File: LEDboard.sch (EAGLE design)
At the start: 307 parts, among them IC1 REG1117, Q1 MMUN2133LT1G, U1 IS31FL3741_QFN60, U2 IS31FL3741_QFN60, U3 ATSAMD21G-A, U4 TPS61090RSAR, U5 MCP73831T-2ACI/OT

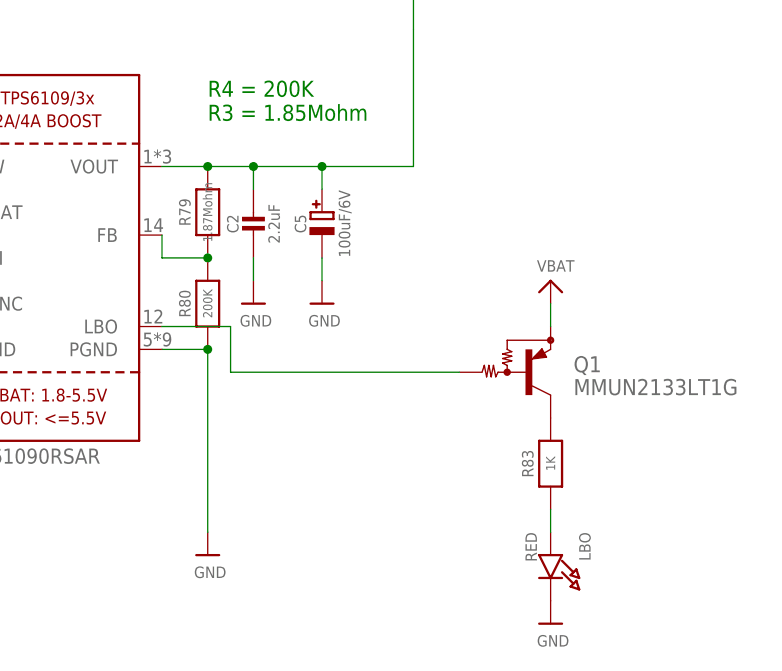
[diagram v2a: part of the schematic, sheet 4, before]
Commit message: Remove LBO, change bypass cap
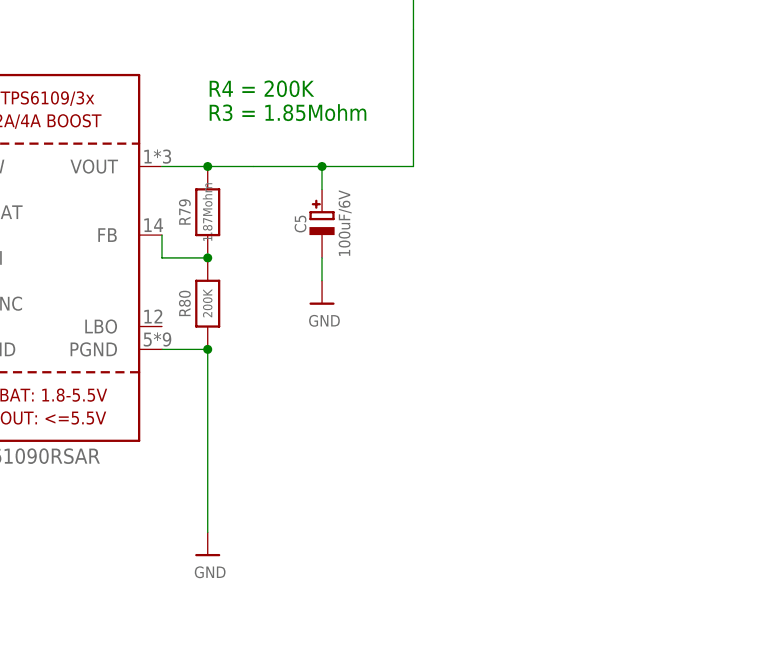
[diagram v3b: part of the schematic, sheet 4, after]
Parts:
- removed C2: 2.2uF, microbuilder:CAP_CERAMIC0805-NOOUTLINE
- removed LBO: RED, microbuilder:LED0805_NOOUTLINE
- removed Q1: MMUN2133LT1G, transistor:MUN2114T1-PNP_DRIVER-SC59-BEC
- removed R83: 1K, microbuilder:RESISTOR0805_NOOUTLINE
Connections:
- removed net LBO: Q1.B, U4.LBO
- removed net N$77: LBO.A, R83.1
- removed net N$78: Q1.C, R83.2
- net 5.0V: no longer C2.1
- net GND: no longer C2.2, LBO.C
- net VBAT: no longer Q1.E
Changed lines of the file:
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@@
 <part name="B1" library="microbuilder" deviceset="BATTERY" device="" value="S2B-PH-SM4-TB(LF)(SN)"/>
 <part name="U$5" library="microbuilder" deviceset="GND" device=""/>
-<part name="C2" library="microbuilder" deviceset="CAP_CERAMIC" device="0805-NOOUTLINE" value="2.2uF"/>
 <part name="U$7" library="microbuilder" deviceset="5.0V" device=""/>
 <part name="U$19" library="microbuilder" deviceset="VBAT" device=""/>
@@
 <part name="R80" library="microbuilder" deviceset="RESISTOR" device="0805_NOOUTLINE" value="200K"/>
 <part name="U$3" library="microbuilder" deviceset="GND" device=""/>
-<part name="U$6" library="microbuilder" deviceset="GND" device=""/>
 <part name="U$8" library="microbuilder" deviceset="GND" device=""/>
 <part name="R81" library="microbuilder" deviceset="RESISTOR" device="0805_NOOUTLINE" value="340K"/>
 <part name="R82" library="microbuilder" deviceset="RESISTOR" device="0805_NOOUTLINE" value="1.87Mohm"/>
 <part name="C5" library="microbuilder" deviceset="CAP_TANTALUM" device="B/3528_REFLOW" value="100uF/6V"/>
-<part name="LBO" library="microbuilder" deviceset="LED" device="0805_NOOUTLINE" value="RED"/>
-<part name="R83" library="microbuilder" deviceset="RESISTOR" device="0805_NOOUTLINE" value="1K"/>
-<part name="U$20" library="microbuilder" deviceset="GND" device=""/>
-<part name="U$11" library="microbuilder" deviceset="VBAT" device=""/>
-<part name="Q1" library="transistor" deviceset="*-PNP_DRIVER-" device="SC59-BEC" technology="MUN2114T1" value="MMUN2133LT1G"/>
 <part name="U5" library="microbuilder" deviceset="MCP73831/2" device="" value="MCP73831T-2ACI/OT"/>
 <part name="LED3" library="microbuilder" deviceset="LED" device="0805_NOOUTLINE" value="ORANGE"/>
@@
 <instance part="B1" gate="G$1" x="22.86" y="55.88" rot="R90"/>
 <instance part="U$5" gate="G$1" x="22.86" y="48.26"/>
-<instance part="C2" gate="G$1" x="106.68" y="60.96"/>
 <instance part="U$7" gate="G$1" x="124.46" y="91.44"/>
 <instance part="U$19" gate="G$1" x="38.1" y="73.66"/>
@@
 <instance part="R80" gate="G$1" x="101.6" y="53.34" rot="R90"/>
 <instance part="U$3" gate="G$1" x="101.6" y="25.4"/>
-<instance part="U$6" gate="G$1" x="106.68" y="53.34"/>
 <instance part="U$8" gate="G$1" x="114.3" y="53.34"/>
 <instance part="R81" gate="G$1" x="53.34" y="35.56" rot="R90"/>
 <instance part="R82" gate="G$1" x="53.34" y="58.42" rot="R90"/>
 <instance part="C5" gate="G$1" x="114.3" y="60.96"/>
-<instance part="LBO" gate="G$1" x="139.7" y="22.86" rot="R270"/>
-<instance part="R83" gate="G$1" x="139.7" y="35.56" rot="R90"/>
-<instance part="U$20" gate="G$1" x="139.7" y="17.78"/>
-<instance part="U$11" gate="G$1" x="139.7" y="55.88"/>
-<instance part="Q1" gate="G$1" x="137.16" y="45.72" smashed="yes">
-<attribute name="NAME" x="142.24" y="45.72" size="1.778" layer="95"/>
-<attribute name="VALUE" x="142.24" y="43.18" size="1.778" layer="96"/>
-</instance>
 <instance part="U5" gate="G$1" x="114.3" y="127"/>
 <instance part="LED3" gate="G$1" x="81.28" y="124.46"/>
@@
 </segment>
 <segment>
-<pinref part="C2" gate="G$1" pin="2"/>
-<wire x1="106.68" y1="58.42" x2="106.68" y2="55.88" width="0.1524" layer="91"/>
-<pinref part="U$6" gate="G$1" pin="GND"/>
-</segment>
-<segment>
 <wire x1="114.3" y1="58.42" x2="114.3" y2="55.88" width="0.1524" layer="91"/>
 <pinref part="U$8" gate="G$1" pin="GND"/>
@@
 </segment>
 <segment>
-<pinref part="LBO" gate="G$1" pin="C"/>
-<pinref part="U$20" gate="G$1" pin="GND"/>
-</segment>
-<segment>
 <pinref part="U$30" gate="G$1" pin="GND"/>
 <wire x1="50.8" y1="119.38" x2="55.88" y2="119.38" width="0.1524" layer="91"/>
@@
 <wire x1="114.3" y1="68.58" x2="124.46" y2="68.58" width="0.1524" layer="91"/>
 <wire x1="124.46" y1="68.58" x2="124.46" y2="83.82" width="0.1524" layer="91"/>
-<pinref part="C2" gate="G$1" pin="1"/>
 <wire x1="124.46" y1="83.82" x2="124.46" y2="88.9" width="0.1524" layer="91"/>
-<wire x1="106.68" y1="66.04" x2="106.68" y2="68.58" width="0.1524" layer="91"/>
-<junction x="106.68" y="68.58"/>
 <wire x1="114.3" y1="68.58" x2="114.3" y2="66.04" width="0.1524" layer="91"/>
 <junction x="114.3" y="68.58"/>
@@
 </segment>
 <segment>
-<wire x1="139.7" y1="50.8" x2="139.7" y2="53.34" width="0.1524" layer="91"/>
-<pinref part="U$11" gate="G$1" pin="VBAT"/>
-<pinref part="Q1" gate="G$1" pin="E"/>
-</segment>
-<segment>
 <pinref part="U5" gate="G$1" pin="VBAT"/>
 <wire x1="142.24" y1="129.54" x2="127" y2="129.54" width="0.1524" layer="91"/>
@@
 </segment>
 </net>
-<net name="LBO" class="0">
-<segment>
-<pinref part="U4" gate="G$1" pin="LBO"/>
-<wire x1="96.52" y1="50.8" x2="104.14" y2="50.8" width="0.1524" layer="91"/>
-<wire x1="104.14" y1="50.8" x2="104.14" y2="45.72" width="0.1524" layer="91"/>
-<wire x1="104.14" y1="45.72" x2="129.54" y2="45.72" width="0.1524" layer="91"/>
-<pinref part="Q1" gate="G$1" pin="B"/>
-</segment>
-</net>
-<net name="N$77" class="0">
-<segment>
-<pinref part="LBO" gate="G$1" pin="A"/>
-<pinref part="R83" gate="G$1" pin="1"/>
-<wire x1="139.7" y1="27.94" x2="139.7" y2="30.48" width="0.1524" layer="91"/>
-</segment>
-</net>
-<net name="N$78" class="0">
-<segment>
-<pinref part="R83" gate="G$1" pin="2"/>
-<pinref part="Q1" gate="G$1" pin="C"/>
-</segment>
-</net>

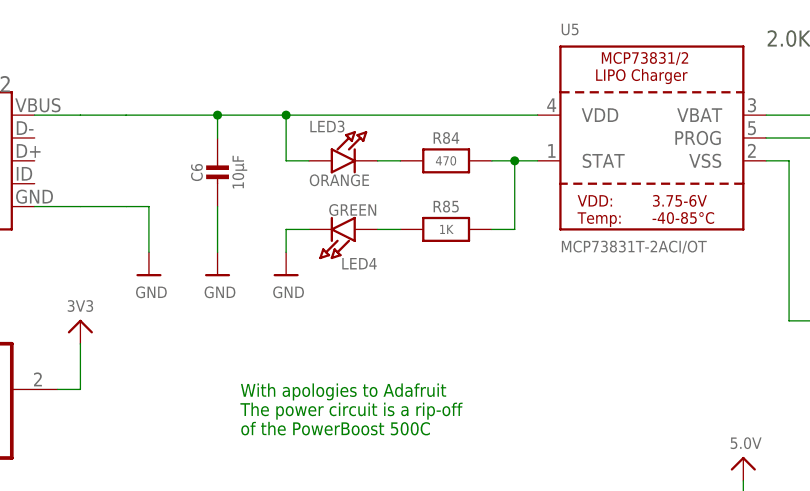
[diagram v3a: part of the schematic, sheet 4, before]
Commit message: holy shit one layer
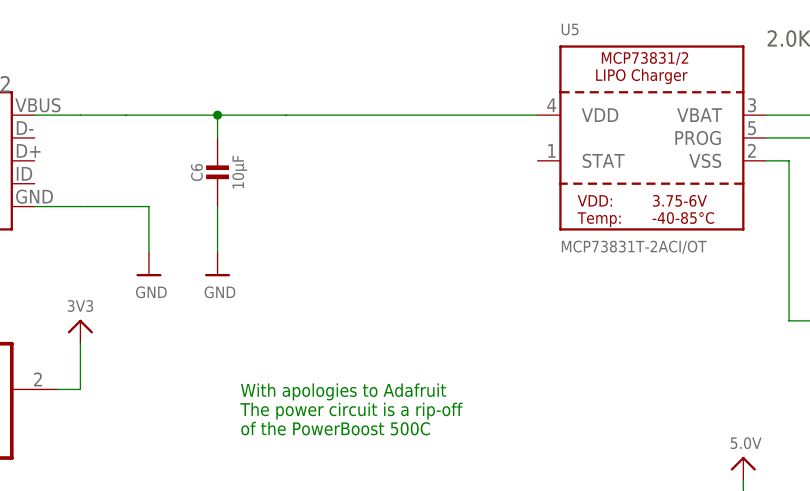
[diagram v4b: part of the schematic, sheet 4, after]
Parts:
- removed LED3: ORANGE, microbuilder:LED0805_NOOUTLINE
- removed LED4: GREEN, microbuilder:LED0805_NOOUTLINE
- removed R84: 470, microbuilder:RESISTOR0805_NOOUTLINE
- removed R85: 1K, microbuilder:RESISTOR0805_NOOUTLINE
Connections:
- removed net N$79: LED3.C, R84.1
- removed net N$80: R84.2, R85.2, U5.STAT
- removed net N$82: LED4.A, R85.1
- net GND: no longer LED4.C
- net VDD1: no longer LED3.A
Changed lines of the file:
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@@
 <part name="C5" library="microbuilder" deviceset="CAP_TANTALUM" device="B/3528_REFLOW" value="100uF/6V"/>
 <part name="U5" library="microbuilder" deviceset="MCP73831/2" device="" value="MCP73831T-2ACI/OT"/>
-<part name="LED3" library="microbuilder" deviceset="LED" device="0805_NOOUTLINE" value="ORANGE"/>
-<part name="LED4" library="microbuilder" deviceset="LED" device="0805_NOOUTLINE" value="GREEN"/>
-<part name="R84" library="microbuilder" deviceset="RESISTOR" device="0805_NOOUTLINE" value="470"/>
-<part name="R85" library="microbuilder" deviceset="RESISTOR" device="0805_NOOUTLINE" value="1K"/>
 <part name="U$30" library="microbuilder" deviceset="GND" device=""/>
 <part name="C6" library="microbuilder" deviceset="CAP_CERAMIC" device="0805-NOOUTLINE" value="10µF"/>
@@
 <part name="R86" library="microbuilder" deviceset="RESISTOR" device="0805_NOOUTLINE" value="2k"/>
 <part name="U$32" library="microbuilder" deviceset="GND" device=""/>
-<part name="U$33" library="microbuilder" deviceset="GND" device=""/>
 <part name="U$34" library="microbuilder" deviceset="VBAT" device=""/>
 <part name="J2" library="SparkFun-Connectors" library_urn="urn:adsk.eagle:library:513" deviceset="USB_MICRO-B" device="_FEMALE-SMT" package3d_urn="urn:adsk.eagle:package:38238/1"/>
@@
 <instance part="C5" gate="G$1" x="114.3" y="60.96"/>
 <instance part="U5" gate="G$1" x="114.3" y="127"/>
-<instance part="LED3" gate="G$1" x="81.28" y="124.46"/>
-<instance part="LED4" gate="G$1" x="78.74" y="116.84" rot="R180"/>
-<instance part="R84" gate="G$1" x="91.44" y="124.46"/>
-<instance part="R85" gate="G$1" x="91.44" y="116.84"/>
 <instance part="U$30" gate="G$1" x="58.42" y="111.76"/>
 <instance part="C6" gate="G$1" x="66.04" y="121.92"/>
@@
 <instance part="R86" gate="G$1" x="137.16" y="127"/>
 <instance part="U$32" gate="G$1" x="142.24" y="101.6"/>
-<instance part="U$33" gate="G$1" x="73.66" y="111.76"/>
 <instance part="U$34" gate="G$1" x="142.24" y="132.08"/>
 <instance part="J2" gate="G$1" x="40.64" y="124.46" rot="MR0"/>
@@
 </segment>
 <segment>
-<pinref part="U$33" gate="G$1" pin="GND"/>
-<wire x1="73.66" y1="116.84" x2="73.66" y2="114.3" width="0.1524" layer="91"/>
-<pinref part="LED4" gate="G$1" pin="C"/>
-<wire x1="76.2" y1="116.84" x2="73.66" y2="116.84" width="0.1524" layer="91"/>
-</segment>
-<segment>
 <wire x1="35.56" y1="86.36" x2="35.56" y2="83.82" width="0.1524" layer="91"/>
 <pinref part="U$10" gate="G$1" pin="GND"/>
@@
 </segment>
 </net>
-<net name="N$79" class="0">
-<segment>
-<pinref part="LED3" gate="G$1" pin="C"/>
-<pinref part="R84" gate="G$1" pin="1"/>
-<wire x1="83.82" y1="124.46" x2="86.36" y2="124.46" width="0.1524" layer="91"/>
-</segment>
-</net>
-<net name="N$80" class="0">
-<segment>
-<pinref part="R84" gate="G$1" pin="2"/>
-<pinref part="U5" gate="G$1" pin="STAT"/>
-<wire x1="96.52" y1="124.46" x2="99.06" y2="124.46" width="0.1524" layer="91"/>
-<pinref part="R85" gate="G$1" pin="2"/>
-<wire x1="99.06" y1="124.46" x2="101.6" y2="124.46" width="0.1524" layer="91"/>
-<wire x1="96.52" y1="116.84" x2="99.06" y2="116.84" width="0.1524" layer="91"/>
-<wire x1="99.06" y1="116.84" x2="99.06" y2="124.46" width="0.1524" layer="91"/>
-<junction x="99.06" y="124.46"/>
-</segment>
-</net>
 <net name="VDD1" class="0">
 <segment>
@@
 <wire x1="66.04" y1="127" x2="66.04" y2="129.54" width="0.1524" layer="91"/>
 <junction x="66.04" y="129.54"/>
-<pinref part="LED3" gate="G$1" pin="A"/>
-<wire x1="76.2" y1="124.46" x2="73.66" y2="124.46" width="0.1524" layer="91"/>
-<wire x1="73.66" y1="124.46" x2="73.66" y2="129.54" width="0.1524" layer="91"/>
-<junction x="73.66" y="129.54"/>
 <pinref part="J2" gate="G$1" pin="VBUS"/>
 <wire x1="45.72" y1="129.54" x2="50.8" y2="129.54" width="0.1524" layer="91"/>
@@
 </segment>
 </net>
-<net name="N$82" class="0">
-<segment>
-<pinref part="R85" gate="G$1" pin="1"/>
-<pinref part="LED4" gate="G$1" pin="A"/>
-<wire x1="86.36" y1="116.84" x2="83.82" y2="116.84" width="0.1524" layer="91"/>
-</segment>
-</net>

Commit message: micro
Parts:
- removed U3: ATSAMD21G-A, SparkFun-IC-Microcontroller:ATSAMD21G-A
- added C1: 1uF, microbuilder:CAP_CERAMIC0805-NOOUTLINE
- added C2: 0.1uF, microbuilder:CAP_CERAMIC0805-NOOUTLINE
- added C3, C4: 10pF, rcl:C-USC0805
- added MCU: ATSAMD21E, adafruit:ATSAMD21E
- added Y1: 32.768kHz, SparkFun-Clocks:CRYSTAL-32.768KHZSMD-3.2X1.5
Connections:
- new net D+: J2.D+, MCU.D+
- new net D-: J2.D-, MCU.D-
- new net N$75: C1.2, MCU.VCORE
- new net N$77: C2.2, MCU.VDD
- new net N$78: C4.1, MCU.PA1, Y1.1
- new net N$79: C3.1, MCU.PA0, Y1.2
- new net RESET: MCU.RESET
- new net SWCLK: MCU.SWCLK
- new net SWDIO: MCU.SWDIO
- net 3V3: now also C1.1, C2.1
- net GND: now also C3.2, C4.2, MCU.GND
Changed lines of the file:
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@@
 <part name="R71" library="SparkFun-Resistors" library_urn="urn:adsk.eagle:library:532" deviceset="14KOHM" device="-0603-1/10W-1%" package3d_urn="urn:adsk.eagle:package:39650/1" value="20Ω"/>
 <part name="R72" library="SparkFun-Resistors" library_urn="urn:adsk.eagle:library:532" deviceset="14KOHM" device="-0603-1/10W-1%" package3d_urn="urn:adsk.eagle:package:39650/1" value="20Ω"/>
-<part name="U3" library="SparkFun-IC-Microcontroller" library_urn="urn:adsk.eagle:library:525" deviceset="ATSAMD21G" device="-A" package3d_urn="urn:adsk.eagle:package:38963/1"/>
 <part name="U4" library="microbuilder" deviceset="VREG_TPS6103X" device="" value="TPS61090RSAR"/>
 <part name="L1" library="microbuilder" deviceset="INDUCTOR" device="TDK_VLC5045" value="VLC5045-6.8uH"/>
@@
 <part name="U$12" library="microbuilder" deviceset="5.0V" device=""/>
 <part name="U$13" library="microbuilder" deviceset="5.0V" device="" value="3V3"/>
+<part name="MCU" library="adafruit" deviceset="ATSAMD21E" device=""/>
+<part name="U$6" library="microbuilder" deviceset="5.0V" device="" value="3V3"/>
+<part name="C1" library="microbuilder" deviceset="CAP_CERAMIC" device="0805-NOOUTLINE" value="1uF"/>
+<part name="U$9" library="microbuilder" deviceset="GND" device=""/>
+<part name="C2" library="microbuilder" deviceset="CAP_CERAMIC" device="0805-NOOUTLINE" value="0.1uF"/>
+<part name="Y1" library="SparkFun-Clocks" library_urn="urn:adsk.eagle:library:511" deviceset="CRYSTAL-32.768KHZ" device="SMD-3.2X1.5" package3d_urn="urn:adsk.eagle:package:37548/1" value="32.768kHz"/>
+<part name="U$11" library="microbuilder" deviceset="GND" device=""/>
+<part name="C3" library="rcl" library_urn="urn:adsk.eagle:library:334" deviceset="C-US" device="C0805" package3d_urn="urn:adsk.eagle:package:23617/2" value="10pF"/>
+<part name="C4" library="rcl" library_urn="urn:adsk.eagle:library:334" deviceset="C-US" device="C0805" package3d_urn="urn:adsk.eagle:package:23617/2" value="10pF"/>
 </parts>
 <sheets>
@@
 </plain>
 <instances>
-<instance part="U3" gate="G$1" x="40.64" y="38.1"/>
+<instance part="MCU" gate="G$1" x="50.8" y="48.26"/>
+<instance part="U$6" gate="G$1" x="22.86" y="81.28"/>
+<instance part="C1" gate="G$1" x="27.94" y="66.04" rot="R90"/>
+<instance part="U$9" gate="G$1" x="22.86" y="10.16"/>
+<instance part="C2" gate="G$1" x="30.48" y="71.12" rot="R90"/>
+<instance part="Y1" gate="G$1" x="78.74" y="50.8" rot="R180"/>
+<instance part="U$11" gate="G$1" x="78.74" y="35.56"/>
+<instance part="C3" gate="G$1" x="73.66" y="45.72"/>
+<instance part="C4" gate="G$1" x="83.82" y="45.72"/>
 </instances>
 <busses>
 </busses>
 <nets>
+<net name="D-" class="0">
+<segment>
+<pinref part="MCU" gate="G$1" pin="D-"/>
+<wire x1="33.02" y1="35.56" x2="22.86" y2="35.56" width="0.1524" layer="91"/>
+<label x="22.86" y="35.56" size="1.778" layer="95"/>
+</segment>
+</net>
+<net name="D+" class="0">
+<segment>
+<pinref part="MCU" gate="G$1" pin="D+"/>
+<wire x1="33.02" y1="38.1" x2="22.86" y2="38.1" width="0.1524" layer="91"/>
+<label x="22.86" y="38.1" size="1.778" layer="95"/>
+</segment>
+</net>
+<net name="3V3" class="0">
+<segment>
+<pinref part="U$6" gate="G$1" pin="5.0V"/>
+<wire x1="22.86" y1="73.66" x2="22.86" y2="78.74" width="0.1524" layer="91"/>
+<wire x1="22.86" y1="71.12" x2="22.86" y2="73.66" width="0.1524" layer="91"/>
+<pinref part="C1" gate="G$1" pin="1"/>
+<wire x1="22.86" y1="66.04" x2="22.86" y2="71.12" width="0.1524" layer="91"/>
+<pinref part="C2" gate="G$1" pin="1"/>
+<wire x1="25.4" y1="71.12" x2="22.86" y2="71.12" width="0.1524" layer="91"/>
+<junction x="22.86" y="71.12"/>
+</segment>
+</net>
+<net name="N$75" class="0">
+<segment>
+<pinref part="MCU" gate="G$1" pin="VCORE"/>
+<pinref part="C1" gate="G$1" pin="2"/>
+<wire x1="33.02" y1="66.04" x2="30.48" y2="66.04" width="0.1524" layer="91"/>
+</segment>
+</net>
+<net name="GND" class="0">
+<segment>
+<wire x1="22.86" y1="15.24" x2="22.86" y2="12.7" width="0.1524" layer="91"/>
+<pinref part="U$9" gate="G$1" pin="GND"/>
+<pinref part="MCU" gate="G$1" pin="GND"/>
+<wire x1="33.02" y1="15.24" x2="22.86" y2="15.24" width="0.1524" layer="91"/>
+</segment>
+<segment>
+<wire x1="78.74" y1="40.64" x2="78.74" y2="38.1" width="0.1524" layer="91"/>
+<pinref part="U$11" gate="G$1" pin="GND"/>
+<pinref part="C3" gate="G$1" pin="2"/>
+<wire x1="73.66" y1="40.64" x2="78.74" y2="40.64" width="0.1524" layer="91"/>
+<pinref part="C4" gate="G$1" pin="2"/>
+<wire x1="83.82" y1="40.64" x2="78.74" y2="40.64" width="0.1524" layer="91"/>
+<junction x="78.74" y="40.64"/>
+</segment>
+</net>
+<net name="N$77" class="0">
+<segment>
+<pinref part="C2" gate="G$1" pin="2"/>
+<pinref part="MCU" gate="G$1" pin="VDD"/>
+</segment>
+</net>
+<net name="N$78" class="0">
+<segment>
+<pinref part="MCU" gate="G$1" pin="PA1"/>
+<wire x1="63.5" y1="53.34" x2="81.28" y2="53.34" width="0.1524" layer="91"/>
+<pinref part="Y1" gate="G$1" pin="1"/>
+<wire x1="81.28" y1="53.34" x2="81.28" y2="50.8" width="0.1524" layer="91"/>
+<pinref part="C4" gate="G$1" pin="1"/>
+<wire x1="83.82" y1="48.26" x2="83.82" y2="53.34" width="0.1524" layer="91"/>
+<wire x1="83.82" y1="53.34" x2="81.28" y2="53.34" width="0.1524" layer="91"/>
+<junction x="81.28" y="53.34"/>
+</segment>
+</net>
+<net name="N$79" class="0">
+<segment>
+<pinref part="MCU" gate="G$1" pin="PA0"/>
+<pinref part="Y1" gate="G$1" pin="2"/>
+<wire x1="63.5" y1="50.8" x2="73.66" y2="50.8" width="0.1524" layer="91"/>
+<pinref part="C3" gate="G$1" pin="1"/>
+<wire x1="73.66" y1="50.8" x2="76.2" y2="50.8" width="0.1524" layer="91"/>
+<wire x1="73.66" y1="48.26" x2="73.66" y2="50.8" width="0.1524" layer="91"/>
+<junction x="73.66" y="50.8"/>
+</segment>
+</net>
+<net name="RESET" class="0">
+<segment>
+<pinref part="MCU" gate="G$1" pin="RESET"/>
+<wire x1="33.02" y1="30.48" x2="17.78" y2="30.48" width="0.1524" layer="91"/>
+<label x="17.78" y="30.48" size="1.778" layer="95"/>
+</segment>
+</net>
+<net name="SWDIO" class="0">
+<segment>
+<pinref part="MCU" gate="G$1" pin="SWDIO"/>
+<wire x1="33.02" y1="25.4" x2="17.78" y2="25.4" width="0.1524" layer="91"/>
+<label x="17.78" y="25.4" size="1.778" layer="95"/>
+</segment>
+</net>
+<net name="SWCLK" class="0">
+<segment>
+<pinref part="MCU" gate="G$1" pin="SWCLK"/>
+<wire x1="33.02" y1="22.86" x2="17.78" y2="22.86" width="0.1524" layer="91"/>
+<label x="17.78" y="22.86" size="1.778" layer="95"/>
+</segment>
+</net>
 </nets>
 </sheet>
@@
 </segment>
 </net>
+<net name="D-" class="0">
+<segment>
+<pinref part="J2" gate="G$1" pin="D-"/>
+<wire x1="45.72" y1="127" x2="58.42" y2="127" width="0.1524" layer="91"/>
+<label x="55.88" y="127" size="1.778" layer="95"/>
+</segment>
+</net>
+<net name="D+" class="0">
+<segment>
+<pinref part="J2" gate="G$1" pin="D+"/>
+<wire x1="45.72" y1="124.46" x2="58.42" y2="124.46" width="0.1524" layer="91"/>
+<label x="55.88" y="124.46" size="1.778" layer="95"/>
+</segment>
+</net>
 </nets>
 </sheet>
@@
 packages will not be understood (or retained) with this version.
 </note>
+<note version="8.4" severity="warning">
+Since Version 8.4, EAGLE supports properties for SPICE simulation.
+Probes in schematics and SPICE mapping objects found in parts and library devices
+will not be understood with this version. Update EAGLE to the latest version
+for full support of SPICE simulation.
+</note>
 </compatibility>
